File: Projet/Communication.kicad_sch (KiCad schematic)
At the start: 3 parts

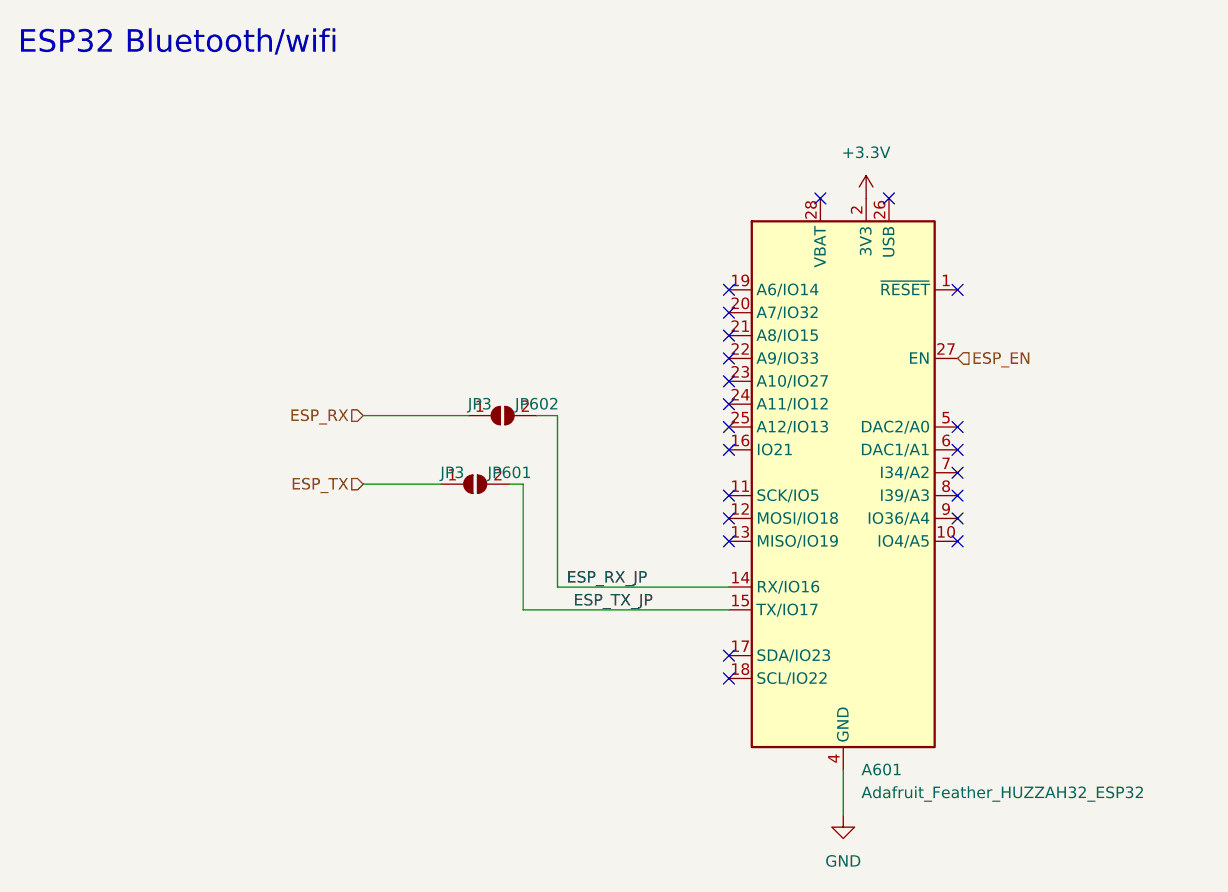
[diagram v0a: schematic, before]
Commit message: PCB_FINAL
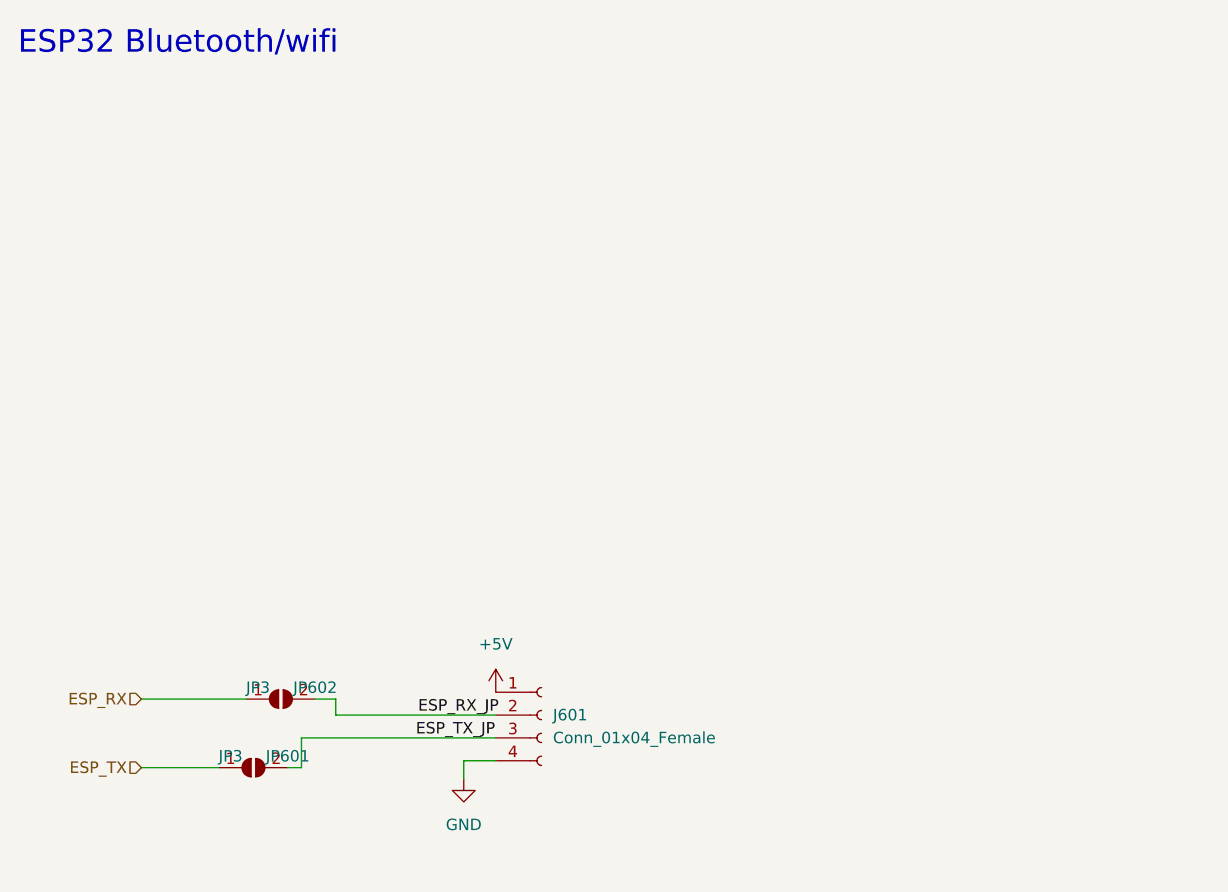
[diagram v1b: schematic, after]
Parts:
- removed A601: Adafruit_Feather_HUZZAH32_ESP32, Module:Adafruit_Feather, symbol MCU_Module:Adafruit_Feather_HUZZAH32_ESP32
- added J601: Conn_01x04_Female, Connector_JST:JST_XH_B4B-XH-A_1x04_P2.50mm_Vertical, symbol Connector:Conn_01x04_Female
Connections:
- net ESP_RX_JP: now also J601.2 (Pin_2)
- net ESP_TX_JP: now also J601.3 (Pin_3)
- net GND: now also J601.4 (Pin_4)
- new net +5V: J601.1 (Pin_1)
- no-connect marks 22 -> 0
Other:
- moved on the sheet: JP601, JP602
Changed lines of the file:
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@@
 (kicad_sch (version 20211123) (generator eeschema)
   (paper "A4")
-  (no_connect (at 104.14 55.88))
-  (no_connect (at 104.14 58.42))
-  (no_connect (at 104.14 60.96))
-  (no_connect (at 104.14 63.5))
-  (no_connect (at 104.14 48.26))
-  (no_connect (at 104.14 50.8))
-  (no_connect (at 104.14 53.34))
-  (no_connect (at 104.14 71.12))
-  (no_connect (at 104.14 73.66))
-  (no_connect (at 104.14 66.04))
-  (no_connect (at 129.54 68.58))
-  (no_connect (at 129.54 76.2))
-  (no_connect (at 129.54 73.66))
-  (no_connect (at 129.54 71.12))
-  (no_connect (at 121.92 38.1))
-  (no_connect (at 114.3 38.1))
-  (no_connect (at 104.14 76.2))
-  (no_connect (at 104.14 88.9))
-  (no_connect (at 104.14 91.44))
-  (no_connect (at 129.54 63.5))
-  (no_connect (at 129.54 48.26))
-  (no_connect (at 129.54 66.04))
-  (wire (pts (xy 104.14 81.28) (xy 85.09 81.28))
+  (wire (pts (xy 47.498 101.346) (xy 38.862 101.346))
     (stroke (width 0) (type default) (color 0 0 0 0))
   )
-  (wire (pts (xy 72.136 69.85) (xy 63.5 69.85))
+  (wire (pts (xy 78.232 98.044) (xy 56.642 98.044))
     (stroke (width 0) (type default) (color 0 0 0 0))
   )
-  (wire (pts (xy 85.09 81.28) (xy 85.09 62.23))
+  (wire (pts (xy 78.232 100.584) (xy 74.676 100.584))
     (stroke (width 0) (type default) (color 0 0 0 0))
   )
-  (wire (pts (xy 75.184 62.23) (xy 63.5 62.23))
+  (wire (pts (xy 60.452 95.504) (xy 60.452 93.726))
     (stroke (width 0) (type default) (color 0 0 0 0))
   )
-  (wire (pts (xy 81.28 83.82) (xy 81.28 69.85))
+  (wire (pts (xy 50.546 93.726) (xy 38.862 93.726))
     (stroke (width 0) (type default) (color 0 0 0 0))
   )
-  (wire (pts (xy 116.84 101.6) (xy 116.84 106.68))
+  (wire (pts (xy 78.232 95.504) (xy 60.452 95.504))
     (stroke (width 0) (type default) (color 0 0 0 0))
   )
-  (wire (pts (xy 81.28 69.85) (xy 79.756 69.85))
+  (wire (pts (xy 56.642 98.044) (xy 56.642 101.346))
     (stroke (width 0) (type default) (color 0 0 0 0))
   )
-  (wire (pts (xy 85.09 62.23) (xy 82.804 62.23))
+  (wire (pts (xy 74.676 100.584) (xy 74.676 102.616))
     (stroke (width 0) (type default) (color 0 0 0 0))
   )
-  (wire (pts (xy 104.14 83.82) (xy 81.28 83.82))
+  (wire (pts (xy 56.642 101.346) (xy 55.118 101.346))
+    (stroke (width 0) (type default) (color 0 0 0 0))
+  )
+  (wire (pts (xy 60.452 93.726) (xy 58.166 93.726))
     (stroke (width 0) (type default) (color 0 0 0 0))
   )
@@
     (effects (font (size 2.5 2.5)) (justify left bottom))
   )
-  (label "ESP_TX_JP" (at 86.868 83.82 0)
+  (label "ESP_TX_JP" (at 69.342 98.044 0)
     (effects (font (size 1.27 1.27)) (justify left bottom))
   )
-  (label "ESP_RX_JP" (at 86.106 81.28 0)
+  (label "ESP_RX_JP" (at 69.596 95.504 0)
     (effects (font (size 1.27 1.27)) (justify left bottom))
   )
-  (hierarchical_label "ESP_EN" (shape input) (at 129.54 55.88 0)
-    (effects (font (size 1.27 1.27)) (justify left))
-  )
-  (hierarchical_label "ESP_TX" (shape input) (at 63.5 69.85 180)
+  (hierarchical_label "ESP_TX" (shape input) (at 38.862 101.346 180)
     (effects (font (size 1.27 1.27)) (justify right))
   )
-  (hierarchical_label "ESP_RX" (shape input) (at 63.5 62.23 180)
+  (hierarchical_label "ESP_RX" (shape input) (at 38.862 93.726 180)
     (effects (font (size 1.27 1.27)) (justify right))
   )
-  (symbol (lib_id "MCU_Module:Adafruit_Feather_HUZZAH32_ESP32") (at 116.84 68.58 0) (unit 1)
+  (symbol (lib_id "power:+5V") (at 78.232 92.964 0) (unit 1)
     (in_bom yes) (on_board yes) (fields_autoplaced)
-    (property "Reference" "A601" (id 0) (at 118.8594 101.6 0)
-      (effects (font (size 1.27 1.27)) (justify left))
-    )
-    (property "Value" "Adafruit_Feather_HUZZAH32_ESP32" (id 1) (at 118.8594 104.14 0)
-      (effects (font (size 1.27 1.27)) (justify left))
-    )
-    (property "Footprint" "Module:Adafruit_Feather" (id 2) (at 119.38 102.87 0)
-      (effects (font (size 1.27 1.27)) (justify left) hide)
-    )
-    (property "Datasheet" "https://cdn-learn.adafruit.com/downloads/pdf/adafruit-huzzah32-esp32-feather.pdf" (id 3) (at 116.84 99.06 0)
+    (property "Reference" "#PWR0121" (id 0) (at 78.232 96.774 0)
       (effects (font (size 1.27 1.27)) hide)
     )
-    (pin "1")
-    (pin "10")
-    (pin "11")
-    (pin "12")
-    (pin "13")
-    (pin "14")
-    (pin "15")
-    (pin "16")
-    (pin "17")
-    (pin "18")
-    (pin "19")
-    (pin "2")
-    (pin "20")
-    (pin "21")
-    (pin "22")
-    (pin "23")
-    (pin "24")
-    (pin "25")
-    (pin "26")
-    (pin "27")
-    (pin "28")
-    (pin "3")
-    (pin "4")
-    (pin "5")
-    (pin "6")
-    (pin "7")
-    (pin "8")
-    (pin "9")
-  )
-  (symbol (lib_id "power:GND") (at 116.84 106.68 0) (unit 1)
-    (in_bom yes) (on_board yes) (fields_autoplaced)
-    (property "Reference" "#PWR0601" (id 0) (at 116.84 113.03 0)
+    (property "Value" "+5V" (id 1) (at 78.232 87.63 0))
+    (property "Footprint" "" (id 2) (at 78.232 92.964 0)
       (effects (font (size 1.27 1.27)) hide)
     )
-    (property "Value" "GND" (id 1) (at 116.84 111.76 0))
-    (property "Footprint" "" (id 2) (at 116.84 106.68 0)
-      (effects (font (size 1.27 1.27)) hide)
-    )
-    (property "Datasheet" "" (id 3) (at 116.84 106.68 0)
+    (property "Datasheet" "" (id 3) (at 78.232 92.964 0)
       (effects (font (size 1.27 1.27)) hide)
     )
     (pin "1")
   )
-  (symbol (lib_id "power:+3.3V") (at 119.38 38.1 0) (unit 1)
+  (symbol (lib_id "power:GND") (at 74.676 102.616 0) (unit 1)
     (in_bom yes) (on_board yes) (fields_autoplaced)
-    (property "Reference" "#PWR0602" (id 0) (at 119.38 41.91 0)
+    (property "Reference" "#PWR0601" (id 0) (at 74.676 108.966 0)
       (effects (font (size 1.27 1.27)) hide)
     )
-    (property "Value" "+3.3V" (id 1) (at 119.38 33.02 0))
-    (property "Footprint" "" (id 2) (at 119.38 38.1 0)
+    (property "Value" "GND" (id 1) (at 74.676 107.696 0))
+    (property "Footprint" "" (id 2) (at 74.676 102.616 0)
       (effects (font (size 1.27 1.27)) hide)
     )
-    (property "Datasheet" "" (id 3) (at 119.38 38.1 0)
+    (property "Datasheet" "" (id 3) (at 74.676 102.616 0)
       (effects (font (size 1.27 1.27)) hide)
     )
     (pin "1")
   )
-  (symbol (lib_id "Jumper:SolderJumper_2_Open") (at 75.946 69.85 0) (unit 1)
+  (symbol (lib_id "Jumper:SolderJumper_2_Open") (at 51.308 101.346 0) (unit 1)
     (in_bom yes) (on_board yes)
-    (property "Reference" "JP601" (id 0) (at 79.756 68.58 0))
-    (property "Value" "JP3" (id 1) (at 73.406 68.58 0))
-    (property "Footprint" "Jumper:SolderJumper-2_P1.3mm_Open_TrianglePad1.0x1.5mm" (id 2) (at 75.946 69.85 0)
+    (property "Reference" "JP601" (id 0) (at 55.118 100.076 0))
+    (property "Value" "JP3" (id 1) (at 48.768 100.076 0))
+    (property "Footprint" "Jumper:SolderJumper-2_P1.3mm_Open_TrianglePad1.0x1.5mm" (id 2) (at 51.308 101.346 0)
       (effects (font (size 1.27 1.27)) hide)
     )
-    (property "Datasheet" "~" (id 3) (at 75.946 69.85 0)
+    (property "Datasheet" "~" (id 3) (at 51.308 101.346 0)
       (effects (font (size 1.27 1.27)) hide)
     )
@@
     (pin "2")
   )
-  (symbol (lib_id "Jumper:SolderJumper_2_Open") (at 78.994 62.23 0) (unit 1)
+  (symbol (lib_id "Jumper:SolderJumper_2_Open") (at 54.356 93.726 0) (unit 1)
     (in_bom yes) (on_board yes)
-    (property "Reference" "JP602" (id 0) (at 82.804 60.96 0))
-    (property "Value" "JP3" (id 1) (at 76.454 60.96 0))
-    (property "Footprint" "Jumper:SolderJumper-2_P1.3mm_Open_TrianglePad1.0x1.5mm" (id 2) (at 78.994 62.23 0)
+    (property "Reference" "JP602" (id 0) (at 58.166 92.456 0))
+    (property "Value" "JP3" (id 1) (at 51.816 92.456 0))
+    (property "Footprint" "Jumper:SolderJumper-2_P1.3mm_Open_TrianglePad1.0x1.5mm" (id 2) (at 54.356 93.726 0)
       (effects (font (size 1.27 1.27)) hide)
     )
-    (property "Datasheet" "~" (id 3) (at 78.994 62.23 0)
+    (property "Datasheet" "~" (id 3) (at 54.356 93.726 0)
       (effects (font (size 1.27 1.27)) hide)
     )
@@
     (pin "2")
   )
+  (symbol (lib_id "Connector:Conn_01x04_Female") (at 83.312 95.504 0) (unit 1)
+    (in_bom yes) (on_board yes) (fields_autoplaced)
+    (property "Reference" "J601" (id 0) (at 84.582 95.5039 0)
+      (effects (font (size 1.27 1.27)) (justify left))
+    )
+    (property "Value" "Conn_01x04_Female" (id 1) (at 84.582 98.0439 0)
+      (effects (font (size 1.27 1.27)) (justify left))
+    )
+    (property "Footprint" "Connector_JST:JST_XH_B4B-XH-A_1x04_P2.50mm_Vertical" (id 2) (at 83.312 95.504 0)
+      (effects (font (size 1.27 1.27)) hide)
+    )
+    (property "Datasheet" "~" (id 3) (at 83.312 95.504 0)
+      (effects (font (size 1.27 1.27)) hide)
+    )
+    (pin "1")
+    (pin "2")
+    (pin "3")
+    (pin "4")
+  )
 )
